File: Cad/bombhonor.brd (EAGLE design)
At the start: 66 x 62.8 mm, 75 parts, among them CN1 HEADER4X1_2MM_SMD, CN2 TR1-01, U1 STM32F030F4

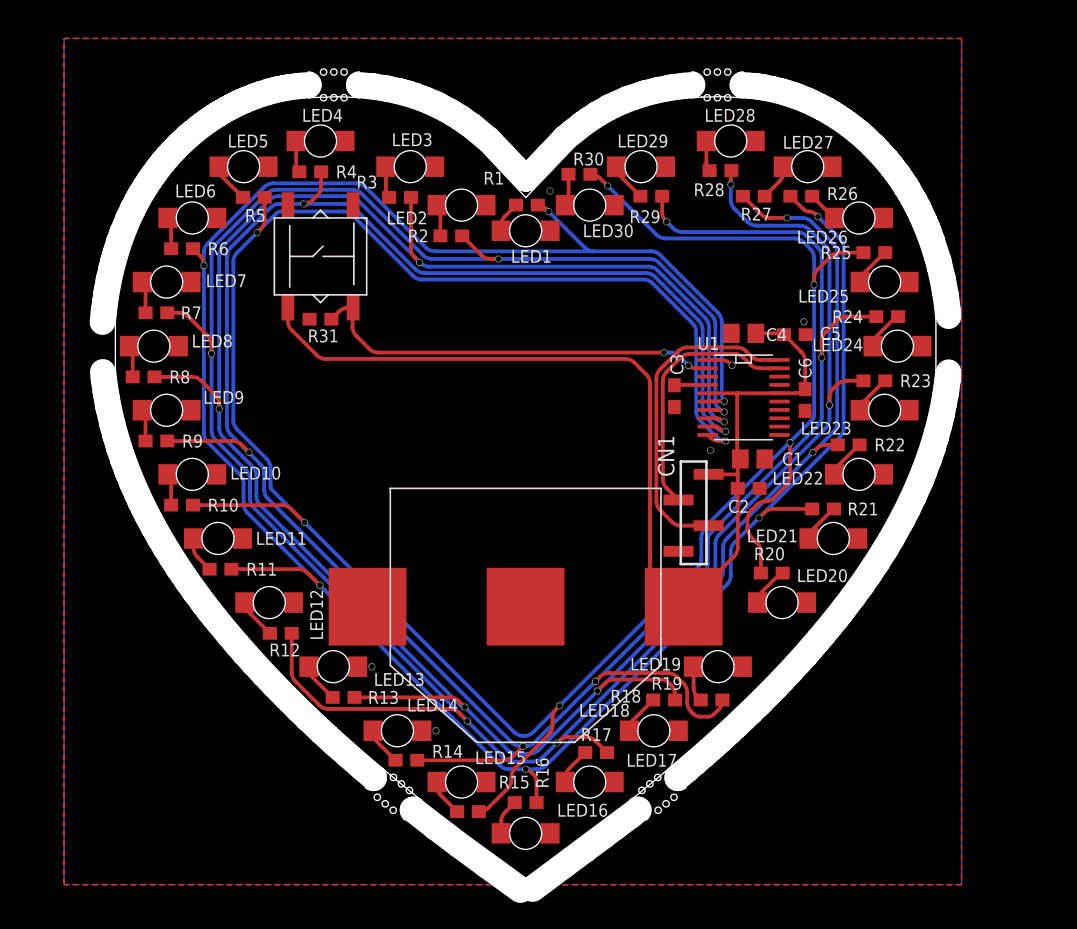
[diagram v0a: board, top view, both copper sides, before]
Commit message: Messe a posto le piste
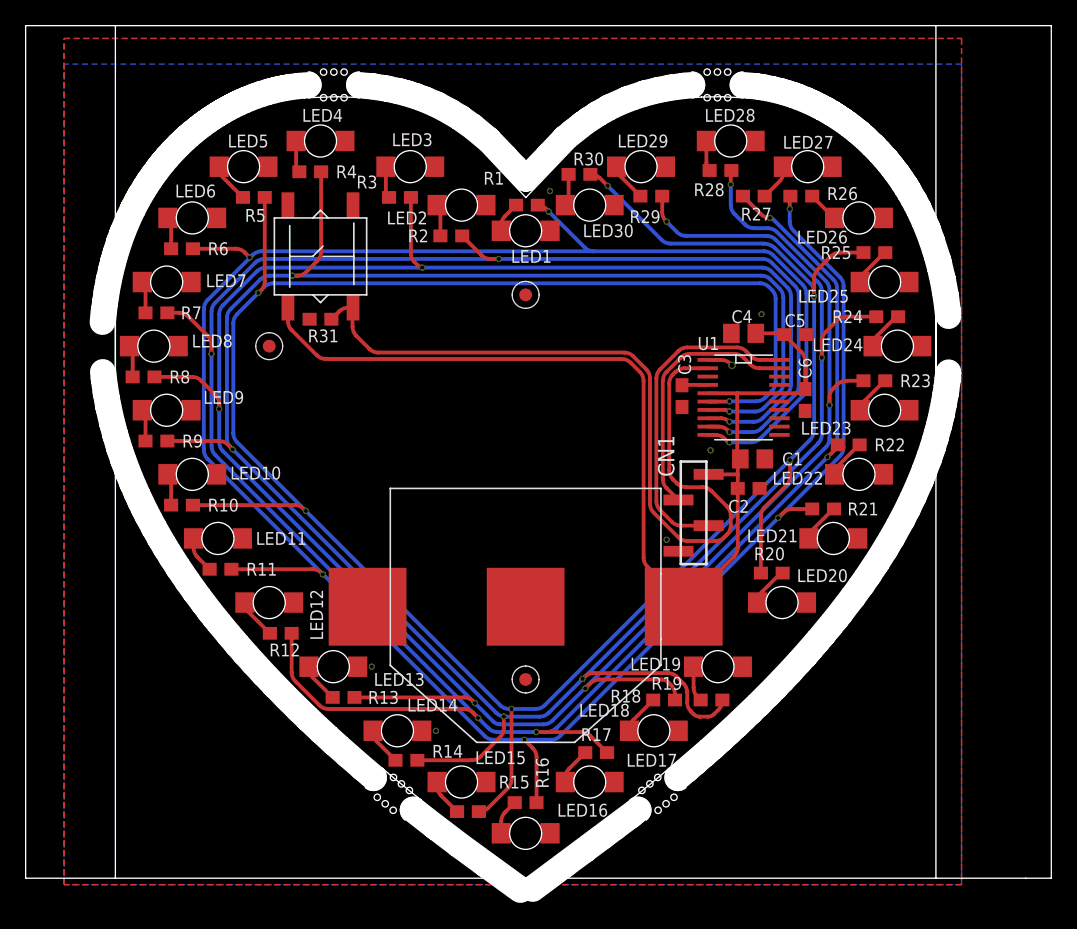
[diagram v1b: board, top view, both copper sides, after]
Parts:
- added U$3, U$4, U$5: (no value), AlmaPANEL:FIDUCIAL_1MM+2MM+CREAM
- moved C3 0.60 mm to (12.2, 6.10)
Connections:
- net LED1: now also U1.10; no longer U1.6
- net LED2: now also U1.9; no longer U1.7
- net LED4: now also U1.7; no longer U1.9
- net LED5: now also U1.6; no longer U1.10
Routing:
- net ON: track 32.5 -> 64.4 mm, vias 2 -> 0
- net LED1: track 185.6 -> 194.5 mm
- net LED5: track 206.5 -> 202.6 mm
- net LED2: track 197.7 -> 201.4 mm
- net LED4: track 202.4 -> 205.0 mm
- net LED3: track 195.9 -> 197.2 mm
- net +3V3: track 86.1 -> 85.3 mm
- net NRST: track 2.61 -> 2.01 mm
- net GND: vias 6 -> 7
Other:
- board size 66 x 62.8 mm -> 80 x 67.4 mm
- board text removed: "C:/Users/lori91et3/Desktop/b.bmp"
